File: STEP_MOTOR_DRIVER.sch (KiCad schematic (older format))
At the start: 1 part

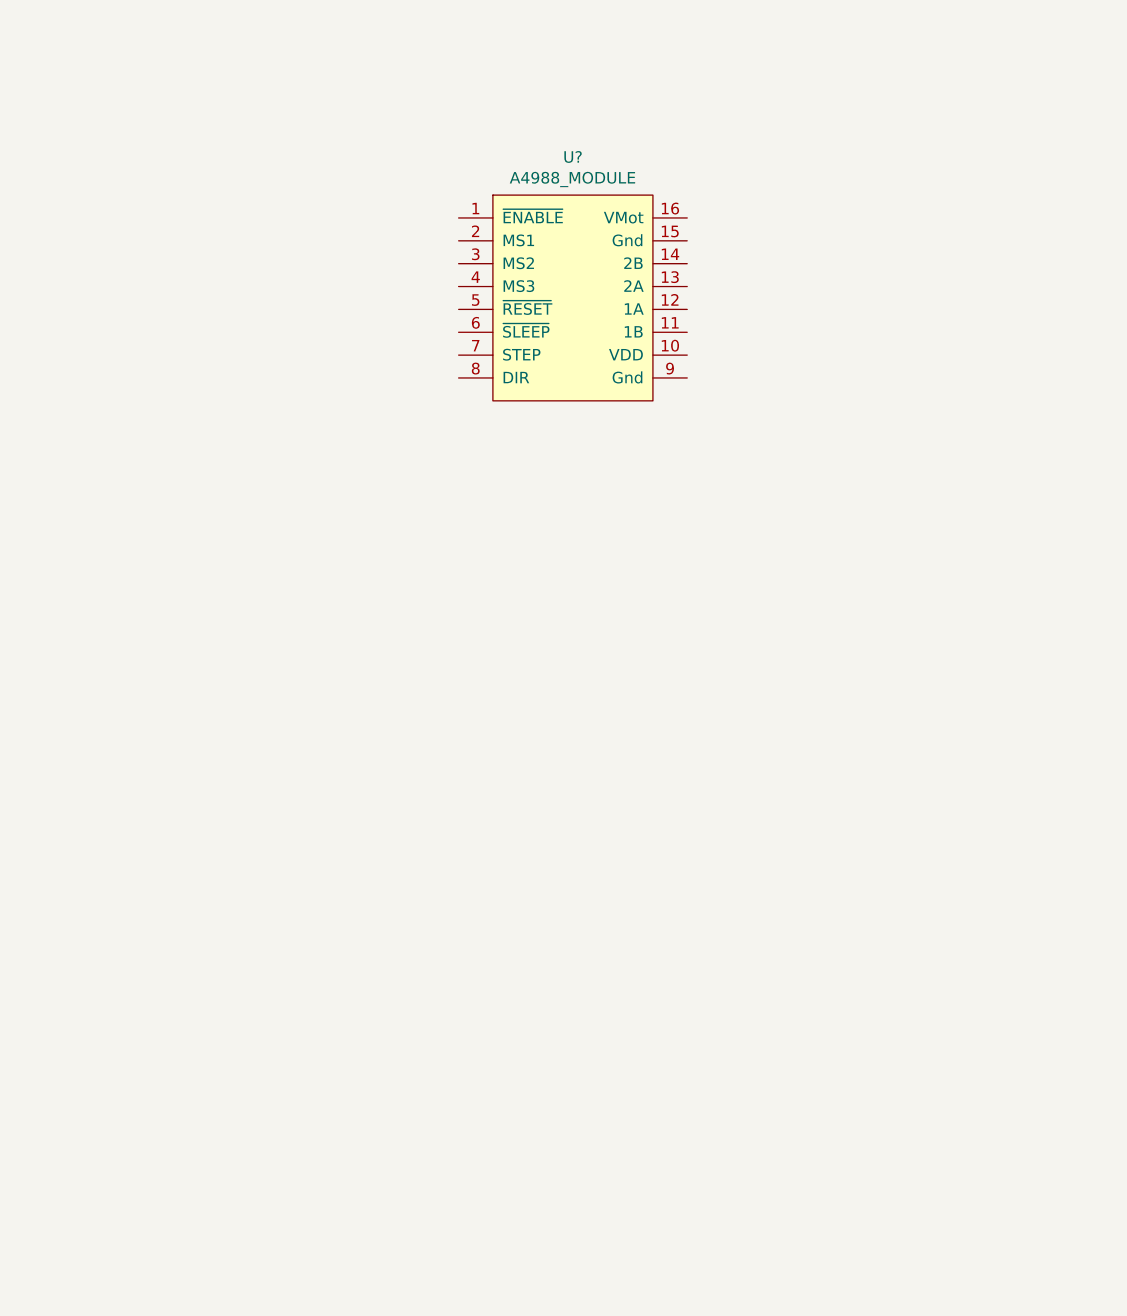
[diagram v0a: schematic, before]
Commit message: update,
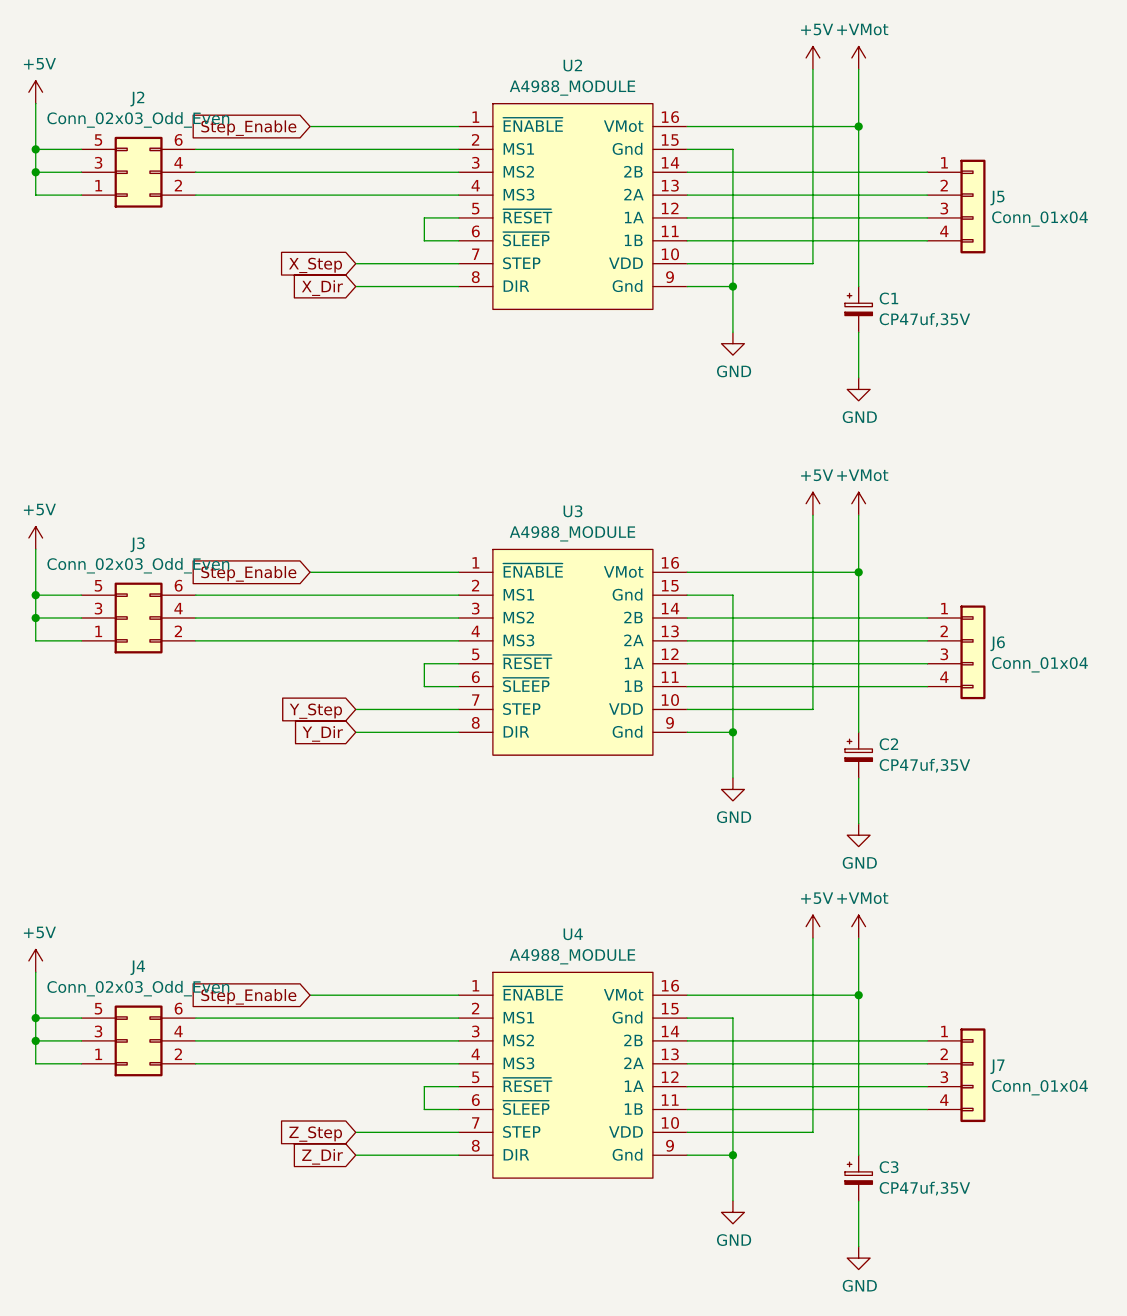
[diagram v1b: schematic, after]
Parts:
- removed U?: A4988_MODULE, symbol taobao-components:A4988_MODULE
- added C1, C2, C3: CP47uf,35V, w_smd_cap:c_elec_5x5.3, symbol taobao-cp:CP47uf,35V
- added J2, J3, J4: Conn_02x03_Odd_Even, Connector_PinHeader_2.54mm:PinHeader_2x03_P2.54mm_Vertical, symbol Connector_Generic:Conn_02x03_Odd_Even
- added J5, J6, J7: Conn_01x04, Connector_PinHeader_2.54mm:PinHeader_1x04_P2.54mm_Vertical, symbol Connector_Generic:Conn_01x04
- added U2, U3, U4: A4988_MODULE, Module:Pololu_Breakout-16_15.2x20.3mm, symbol taobao-components:A4988_MODULE
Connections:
- new net: J2.2 (Pin_2), U2.4 (MS3)
- new net: J2.4 (Pin_4), U2.3 (MS2)
- new net: J2.6 (Pin_6), U2.2 (MS1)
- new net: J5.1 (Pin_1), U2.14 (2B)
- new net: J5.2 (Pin_2), U2.13 (2A)
- new net: J5.3 (Pin_3), U2.12 (1A)
- new net: J5.4 (Pin_4), U2.11 (1B)
- new net: J3.2 (Pin_2), U3.4 (MS3)
- new net: J3.4 (Pin_4), U3.3 (MS2)
- new net: J3.6 (Pin_6), U3.2 (MS1)
- new net: J6.1 (Pin_1), U3.14 (2B)
- new net: J6.2 (Pin_2), U3.13 (2A)
- new net: J6.3 (Pin_3), U3.12 (1A)
- new net: J6.4 (Pin_4), U3.11 (1B)
- new net: J4.2 (Pin_2), U4.4 (MS3)
- new net: J4.4 (Pin_4), U4.3 (MS2)
- new net: J4.6 (Pin_6), U4.2 (MS1)
- new net: J7.1 (Pin_1), U4.14 (2B)
- new net: J7.2 (Pin_2), U4.13 (2A)
- new net: J7.3 (Pin_3), U4.12 (1A)
- new net: J7.4 (Pin_4), U4.11 (1B)
- new net: U2.5 (~RESET~), U2.6 (~SLEEP~)
- new net: U3.5 (~RESET~), U3.6 (~SLEEP~)
- new net: U4.5 (~RESET~), U4.6 (~SLEEP~)
- new net +5V: J2.1 (Pin_1), J2.3 (Pin_3), J2.5 (Pin_5), J3.1 (Pin_1), J3.3 (Pin_3), J3.5 (Pin_5), J4.1 (Pin_1), J4.3 (Pin_3), J4.5 (Pin_5), U2.10 (VDD), U3.10 (VDD), U4.10 (VDD)
- new net +VMot: C1.1, C2.1, C3.1, U2.16 (VMot), U3.16 (VMot), U4.16 (VMot)
- new net GND: C1.2, C2.2, C3.2, U2.15 (Gnd), U2.9 (Gnd), U3.15 (Gnd), U3.9 (Gnd), U4.15 (Gnd), U4.9 (Gnd)
- new net Step_Enable: U2.1 (~ENABLE~), U3.1 (~ENABLE~), U4.1 (~ENABLE~)
- new net X_Dir: U2.8 (DIR)
- new net X_Step: U2.7 (STEP)
- new net Y_Dir: U3.8 (DIR)
- new net Y_Step: U3.7 (STEP)
- new net Z_Dir: U4.8 (DIR)
- new net Z_Step: U4.7 (STEP)

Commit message: update,
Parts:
- J5, J6, J7: footprint Connector_PinHeader_2.54mm:PinHeader_1x04_P2.54mm_Vertical -> Connector_JST:JST_XH_S04B-XH-A-1_1x04_P2.50mm_Horizontal
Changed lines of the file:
@@
 F 0 "J5" H 7830 1642 50  0000 L CNN
 F 1 "Conn_01x04" H 7830 1551 50  0000 L CNN
-F 2 "Connector_PinHeader_2.54mm:PinHeader_1x04_P2.54mm_Vertical" H 7750 1650 50  0001 C CNN
+F 2 "Connector_JST:JST_XH_S04B-XH-A-1_1x04_P2.50mm_Horizontal" H 7750 1650 50  0001 C CNN
 F 3 "~" H 7750 1650 50  0001 C CNN
 	1    7750 1650
@@
 F 0 "J6" H 7830 3592 50  0000 L CNN
 F 1 "Conn_01x04" H 7830 3501 50  0000 L CNN
-F 2 "Connector_PinHeader_2.54mm:PinHeader_1x04_P2.54mm_Vertical" H 7750 3600 50  0001 C CNN
+F 2 "Connector_JST:JST_XH_S04B-XH-A-1_1x04_P2.50mm_Horizontal" H 7750 3600 50  0001 C CNN
 F 3 "~" H 7750 3600 50  0001 C CNN
 	1    7750 3600
@@
 F 0 "J7" H 7830 5442 50  0000 L CNN
 F 1 "Conn_01x04" H 7830 5351 50  0000 L CNN
-F 2 "Connector_PinHeader_2.54mm:PinHeader_1x04_P2.54mm_Vertical" H 7750 5450 50  0001 C CNN
+F 2 "Connector_JST:JST_XH_S04B-XH-A-1_1x04_P2.50mm_Horizontal" H 7750 5450 50  0001 C CNN
 F 3 "~" H 7750 5450 50  0001 C CNN
 	1    7750 5450
